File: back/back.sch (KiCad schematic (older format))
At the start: 16 parts, among them J1 Screw_Terminal_01x02, J2 Screw_Terminal_01x02, J3 Screw_Terminal_01x02, Q1 IRF510, U1 NE555

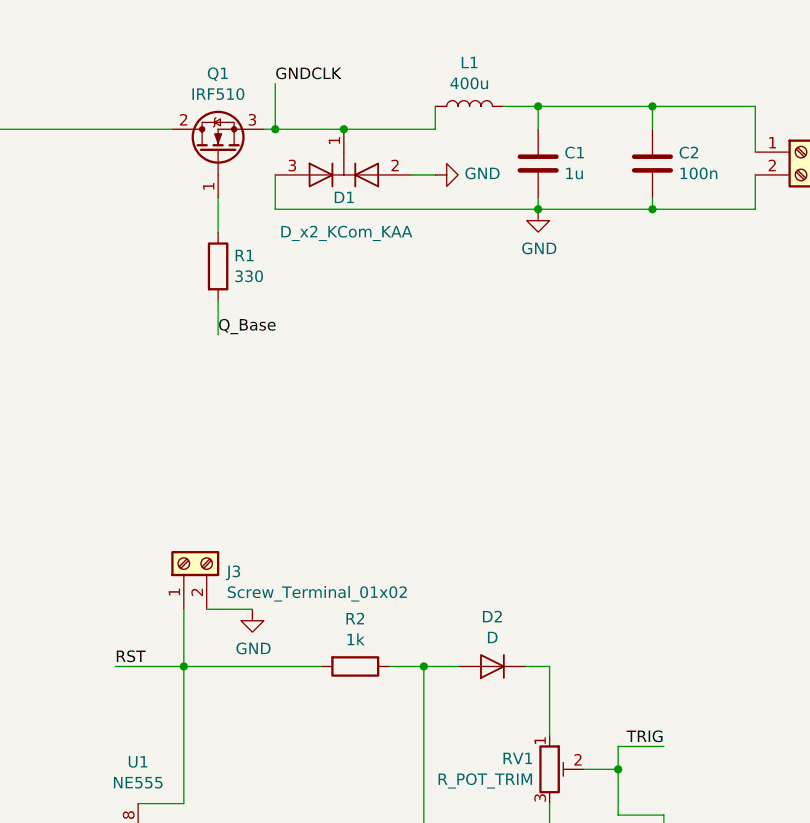
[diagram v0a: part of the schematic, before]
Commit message: wersja nie dzialajaca
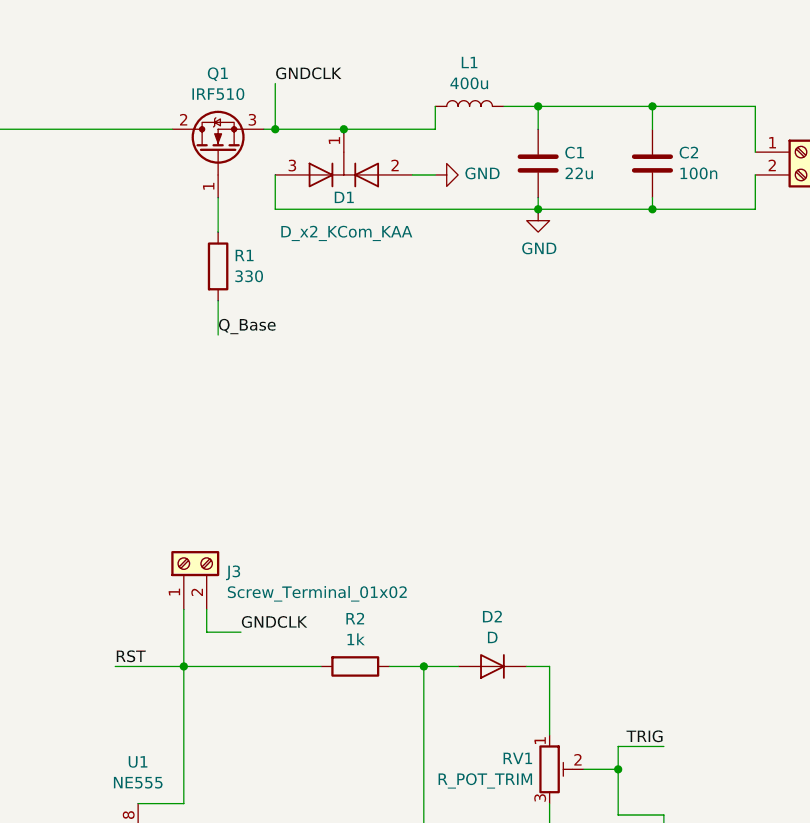
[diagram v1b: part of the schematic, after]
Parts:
- C1: value 1u -> 22u
- U1: footprint Package_DIP:DIP-8_W7.62mm_LongPads -> Package_DIP:DIP-8_W10.16mm_LongPads
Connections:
- net GND: no longer J3.2 (Pin_2)
- net GNDCLK: now also J3.2 (Pin_2)
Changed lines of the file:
@@
-$EndComp
-$Comp
-L Device:C C1
-U 1 1 5CB0B470
-P 4100 1650
-F 0 "C1" H 4215 1696 50  0000 L CNN
-F 1 "1u" H 4215 1605 50  0000 L CNN
-F 2 "Capacitor_THT:CP_Axial_L11.0mm_D5.0mm_P18.00mm_Horizontal" H 4138 1500 50  0001 C CNN
-F 3 "~" H 4100 1650 50  0001 C CNN
-	1    4100 1650
-	1    0    0    -1
 $EndComp
 $Comp
@@
 F 0 "U1" H 2350 5431 50  0000 C CNN
 F 1 "NE555" H 2350 5340 50  0000 C CNN
-F 2 "Package_DIP:DIP-8_W7.62mm_LongPads" H 2350 4850 50  0001 C CNN
+F 2 "Package_DIP:DIP-8_W10.16mm_LongPads" H 2350 4850 50  0001 C CNN
 F 3 "http://www.ti.com/lit/ds/symlink/ne555.pdf" H 2350 4850 50  0001 C CNN
 	1    2350 4850
@@
 RST
 Wire Wire Line
-	2650 3600 2850 3600
-Wire Wire Line
 	1750 5050 1750 5350
 Wire Wire Line
@@
 Wire Wire Line
 	3600 4850 3750 4850
-$Comp
-L power:GND #PWR0102
-U 1 1 5CC493B4
-P 2850 3600
-F 0 "#PWR0102" H 2850 3350 50  0001 C CNN
-F 1 "GND" H 2855 3427 50  0000 C CNN
-F 2 "" H 2850 3600 50  0001 C CNN
-F 3 "" H 2850 3600 50  0001 C CNN
-	1    2850 3600
-	1    0    0    -1
-$EndComp
 $Comp
 L power:GND #PWR0106
@@
 Wire Wire Line
 	4150 4450 4150 4850
+$Comp
+L Device:C C1
+U 1 1 5CB0B470
+P 4100 1650
+F 0 "C1" H 4215 1696 50  0000 L CNN
+F 1 "22u" H 4215 1605 50  0000 L CNN
+F 2 "Capacitor_THT:CP_Axial_L11.0mm_D5.0mm_P18.00mm_Horizontal" H 4138 1500 50  0001 C CNN
+F 3 "~" H 4100 1650 50  0001 C CNN
+	1    4100 1650
+	1    0    0    -1
+$EndComp
+Text Label 2800 3700 0    50   ~ 0
+GNDCLK
+Wire Wire Line
+	2650 3600 2650 3700
+Wire Wire Line
+	2650 3700 2800 3700
 $EndSCHEMATC
